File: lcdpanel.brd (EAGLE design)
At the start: 85 x 56 mm, 31 parts, among them J1 CHARLCD-LONG, SW1 PUSHSW, SW2 PUSHSW, SW3 PUSHSW, SW4 PUSHSW, X1 DCJACK-MJ179P-R

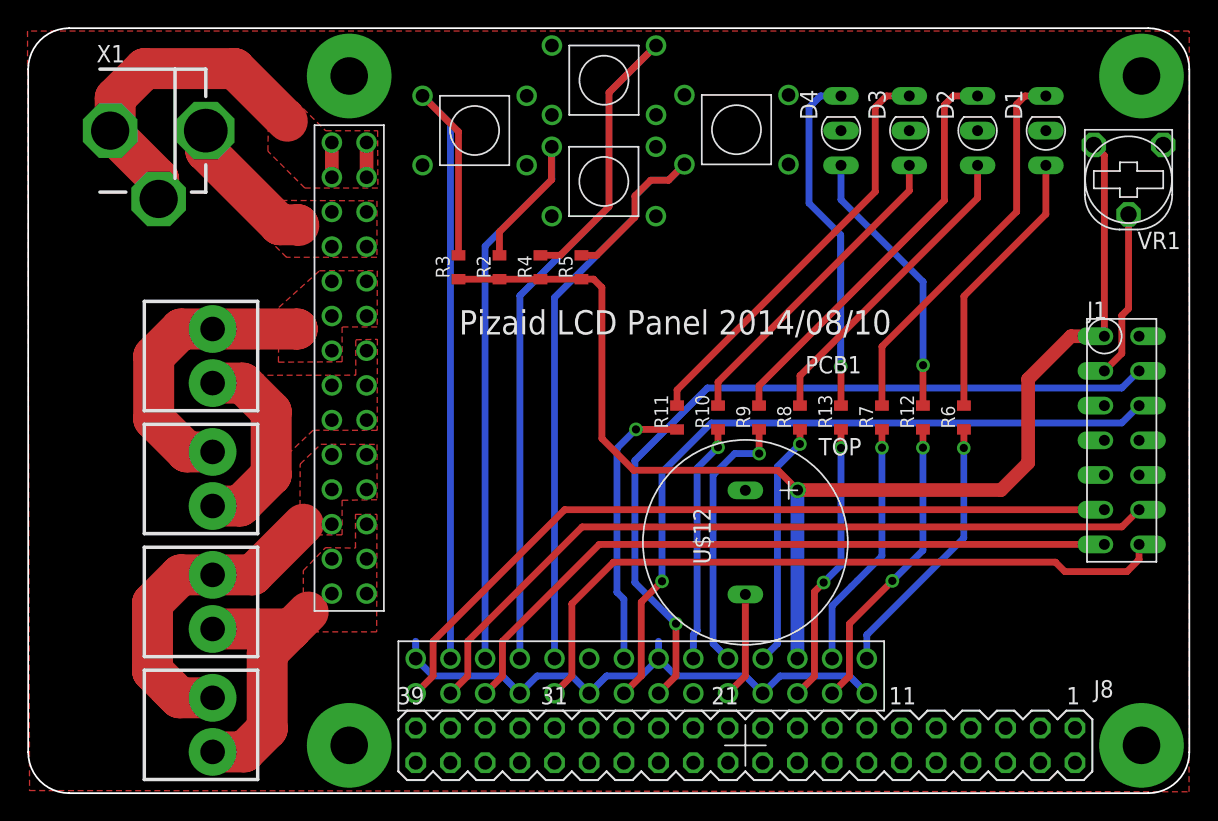
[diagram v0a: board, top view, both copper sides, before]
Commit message: completed rev1
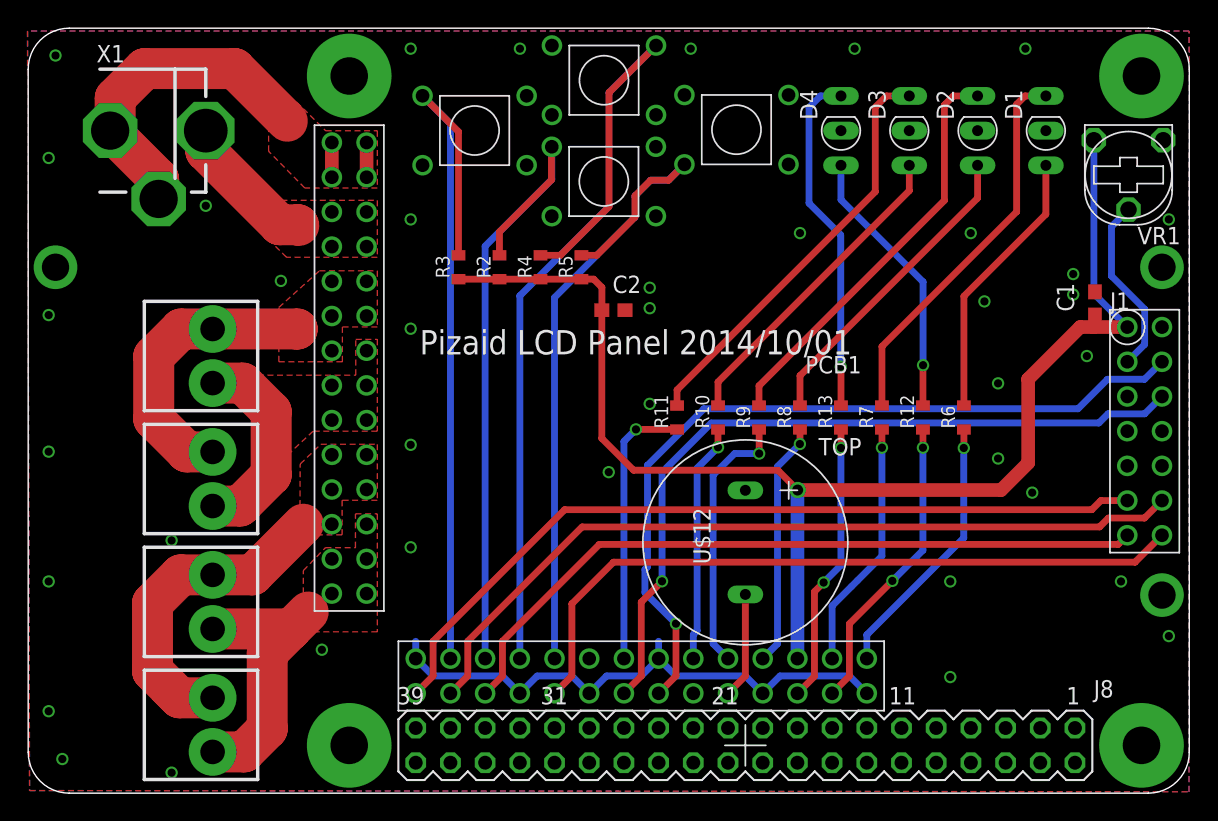
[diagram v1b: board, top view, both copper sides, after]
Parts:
- added C1, C2: (no value), rcl:C0603
- moved J1 1.81 mm to (86.7, 30.5)
- moved VR1 0.35 mm to (85.5, 49.3)
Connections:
- net +5V: now also C1.1, C2.1
- net GND: now also C1.2, C2.2
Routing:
- net +5V: track 95.1 -> 98.3 mm
- net E: track 54.3 -> 56.2 mm
- net DB5: track 57.5 -> 59.4 mm
- net DB6: track 51.3 -> 53.3 mm
- net DB4: track 57.5 -> 59.4 mm
- net N$3: track 12.2 -> 13.2 mm
- net DB7: track 51.6 -> 52.4 mm
- net RS: track 58.4 -> 59.0 mm
- net GND: vias 0 -> 39
- added copper zone on layer 16, net GND
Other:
- board text added: "Pizaid LCD Panel 2014/10/01"
- board text removed: "Pizaid LCD Panel 2014/08/10"
